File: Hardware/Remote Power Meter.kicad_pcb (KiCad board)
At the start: 2 copper layers, 110 x 45 mm, 46 parts, among them J1 USB_C_Receptacle_USB2.0, J2 Conn_01x04_Female, J3 Conn_01x04_Male, J4 Conn_01x02, J5 USB_A, J6 Conn_01x02, J7 Conn_01x04_Male, Q1 UMH3N, SW1 SW_Push, U1 AMS1117-3.3, U2 INA219AxD, U3 CH340C

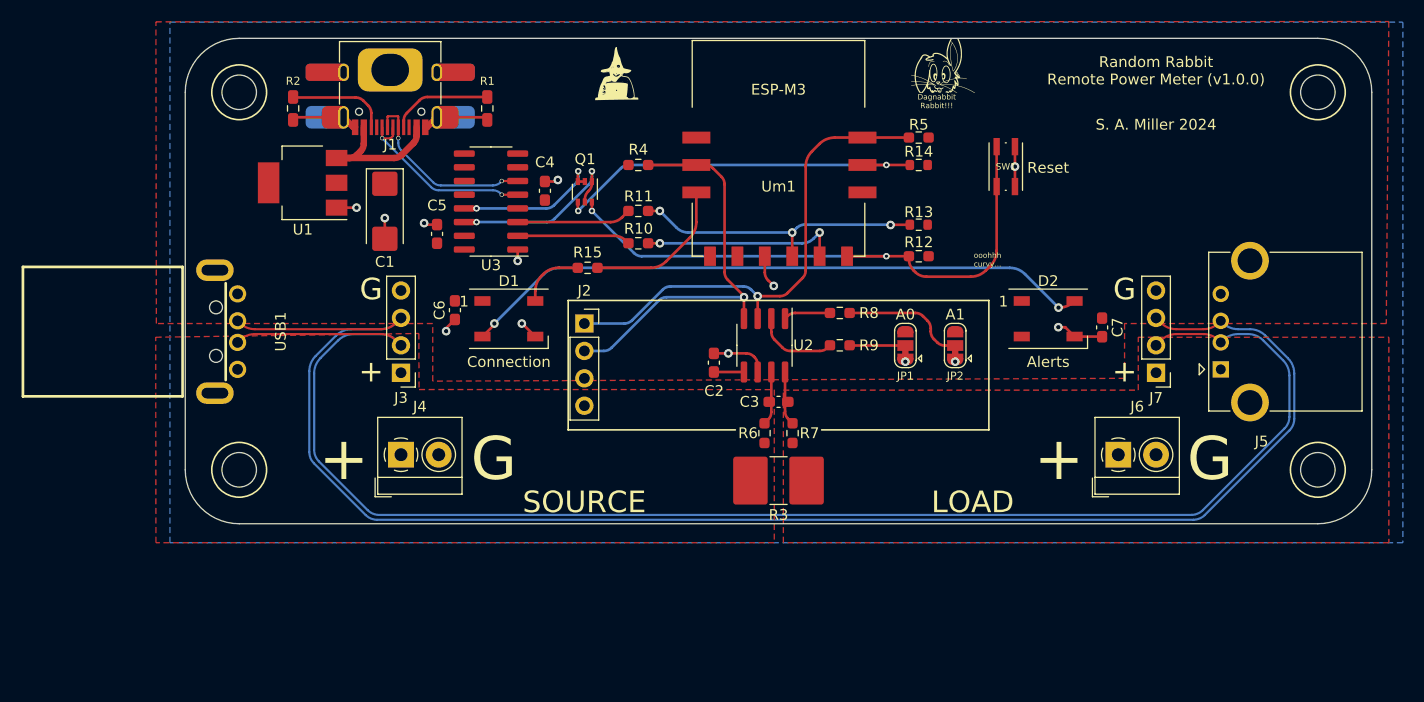
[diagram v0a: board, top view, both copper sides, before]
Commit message: ...
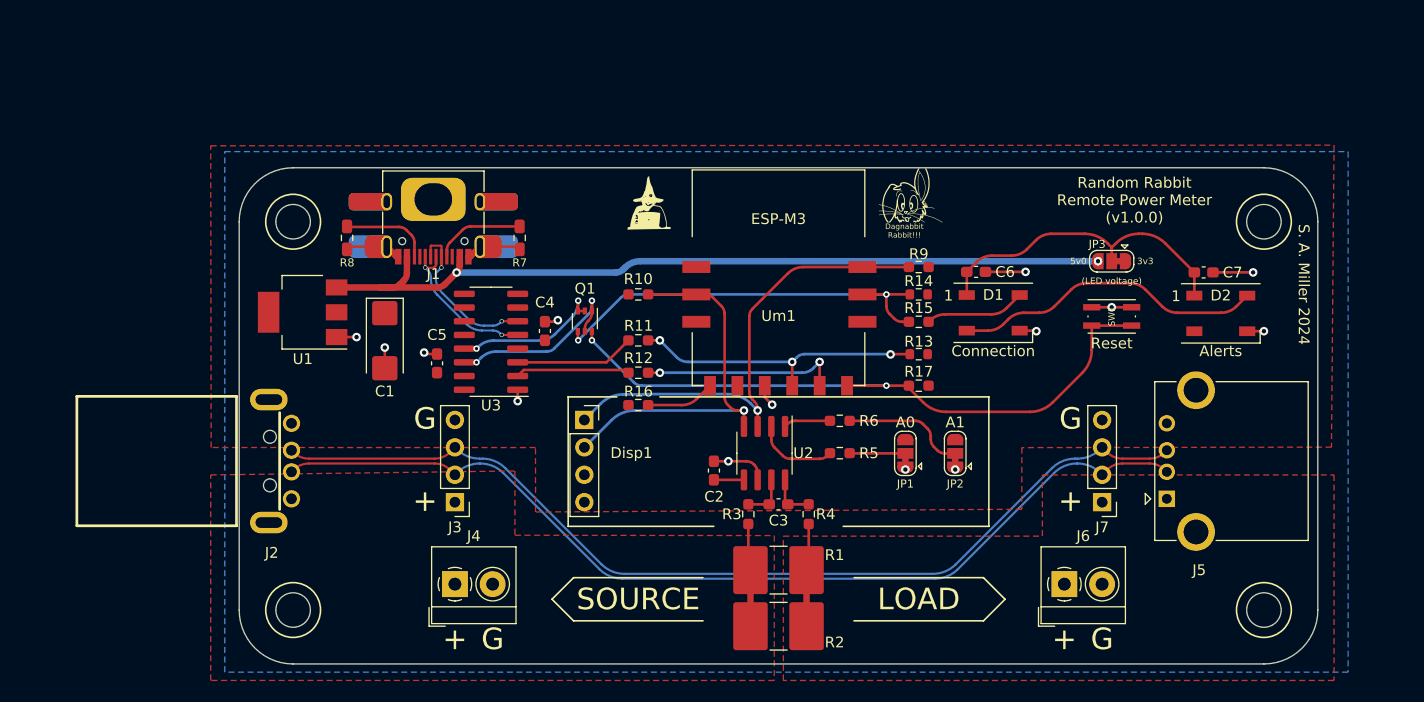
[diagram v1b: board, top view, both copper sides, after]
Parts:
- added JP3: vLED, Jumper:SolderJumper-3_P1.3mm_Bridged12_RoundedPad1.0x1.5mm, F.Cu at (130.9, 85.7)
- added R16: 10K, Resistor_SMD:R_0603_1608Metric_Pad0.98x0.95mm_HandSolder, F.Cu at (87.0, 99.0)
- added R2: 0.1, Resistor_SMD:R_2816_7142Metric_Pad3.20x4.45mm_HandSolder, F.Cu at (100.0, 119.5)
- moved C6 48.4 mm to (118.3, 86.7), turned to 0 degrees
- moved D1 44.9 mm to (119.9, 90.5)
- moved R15 31.1 mm to (113.0, 91.3), turned to 0 degrees
- moved SW1 17.0 mm to (130.9, 90.8), turned to 0 degrees
- moved D2 16.0 mm to (141.0, 90.5)
- moved REF** 13.9 mm to (145.0, 118.0)
- moved REF** 13.9 mm to (55.0, 118.0)
- moved C4 13.0 mm to (78.3, 92.1)
- moved J2 13.0 mm to (53.8, 104.2)
- moved J3 13.0 mm to (70.0, 108.0)
- moved J4 13.0 mm to (70.0, 115.6)
- moved J5 13.0 mm to (136.0, 107.7)
- moved J6 13.0 mm to (126.5, 115.6)
- moved J7 13.0 mm to (130.0, 108.0)
- moved R8 13.0 mm to (60.0, 83.5)
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- renumbered J2 to Disp1, USB1 to J2, R3 to R1, R4 to R10, R10 to R12, R12 to R17, R6 to R3, R7 to R4, R9 to R5, R8 to R6, R1 to R7, R2 to R8, R5 to R9
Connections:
- C6 pad 1: 3v3 -> Net-(C6-Pad1)
- C7 pad 1: 3v3 -> Net-(C6-Pad1)
- D1 pad 1: 3v3 -> Net-(C6-Pad1)
- D2 pad 1: 3v3 -> Net-(C6-Pad1)
- R15 pad 1: IO13 -> IO0
- Um1 pad 4: unconnected-(Um1-Pad4) -> /EN
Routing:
- net Vcc: track 13.9 -> 77.7 mm, vias 0 -> 2
- net D+: track 152.0 -> 91.1 mm
- net D-: track 149.0 -> 91.1 mm
- net Net-(D1-Pad2): track 59.1 -> 28.9 mm, vias 2 -> 0
- net Net-(C6-Pad1): track 0.00 -> 29.9 mm
- net IO13: track 14.0 -> 0.00 mm
- net Vsource: track 0.00 -> 9.56 mm
- net Vload: track 0.00 -> 9.56 mm
- net RST: track 55.8 -> 62.3 mm
- net /EN: track 0.00 -> 6.39 mm
- net IO0: track 35.5 -> 39.4 mm
- net Net-(D1-Pad4): track 6.05 -> 9.28 mm
- net UD+: track 17.5 -> 14.6 mm
- net UD-: track 17.4 -> 15.0 mm
- net I2C SCL: track 37.9 -> 35.7 mm
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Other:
- board size 110 x 45 mm -> 100 x 46 mm
- board text added: "(LED voltage)"
- board text added: "3v3"
- board text added: "5v0"
- board text removed: "ooohhh curvy..."
